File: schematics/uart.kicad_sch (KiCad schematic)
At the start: 4 parts, among them U15 W65C51NxP, Y2 1.8432MHz

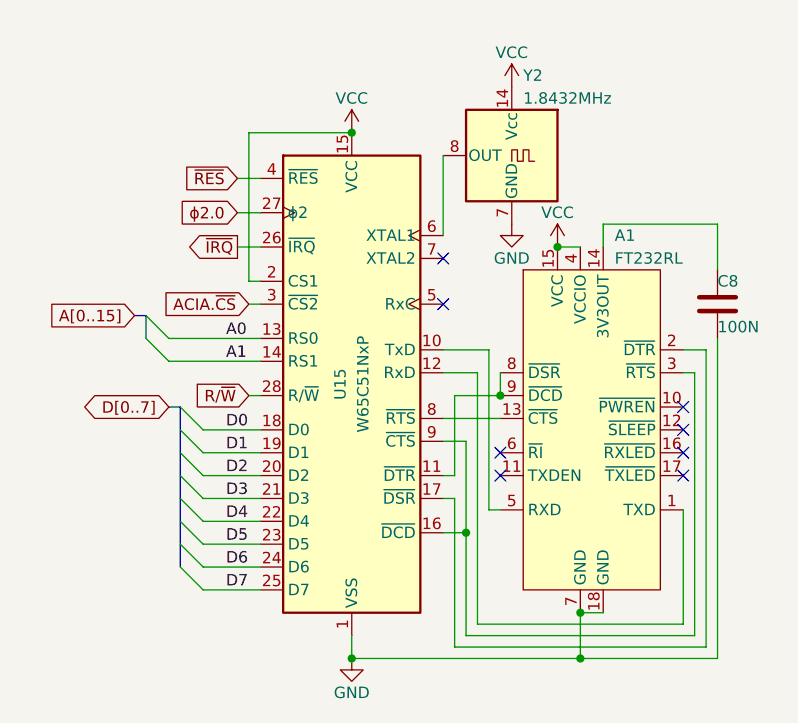
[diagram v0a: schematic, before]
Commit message: ACIA works! Everything works!
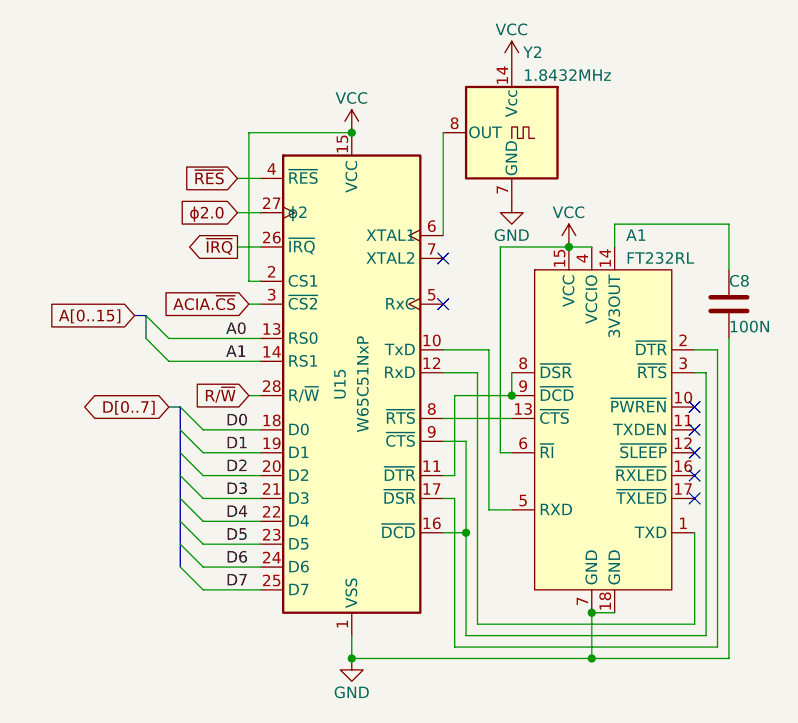
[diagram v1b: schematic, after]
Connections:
- net VCC: now also A1.6 (~{RI})
- no-connect marks 8 -> 7
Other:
- moved on the sheet: A1, C8, Y2
